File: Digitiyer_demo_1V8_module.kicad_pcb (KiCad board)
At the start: 2 copper layers, 37.8 x 35 mm, 104 parts, among them J1 Conn_01x08, J2 Conn_01x24, J3 Conn_01x04_Pin, J4 USB_C_Receptacle_PowerOnly_6P, Q1 AO3400A, Q2 SI1308EDL, U1 Opamp_Quad, U2 LM27762DSSR, U3 TMUX1108PWR, U4 RF-BM-ND05, U5 TPS63900DSKR, U6 TXB0108PWR, U7 74LVC1G34GW, U8 74LVC1G34GW

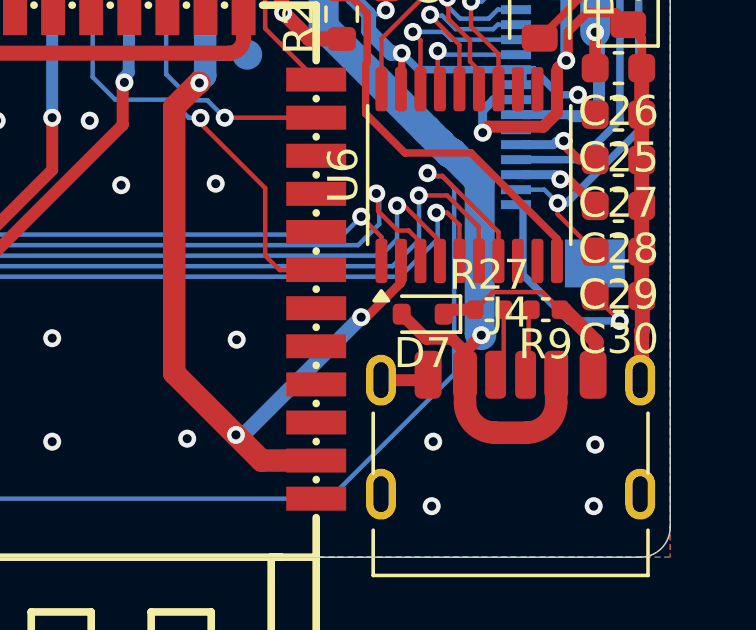
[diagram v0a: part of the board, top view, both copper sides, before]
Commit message: uložit
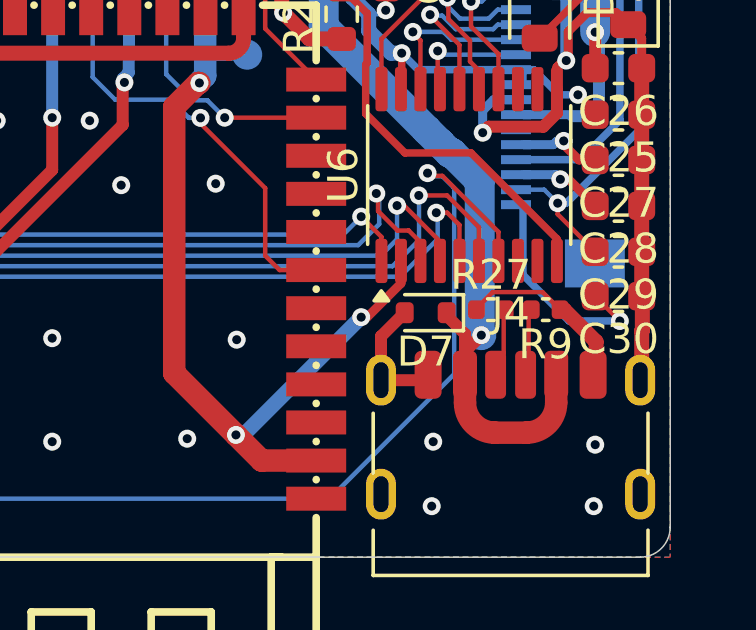
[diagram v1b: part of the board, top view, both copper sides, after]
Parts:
- moved D7 0.11 mm to (181.3, 92.8)
- moved R27 0.05 mm to (183.5, 92.8)
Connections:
- C35 pad 2: Net-(D7-A) -> Net-(D7-C)
- D7 pad 1: GND -> Net-(D7-C)
- D7 pad 2: Net-(D7-A) -> GND
- J4 pad A9: Net-(D7-A) -> Net-(D7-C)
- J4 pad B9: Net-(D7-A) -> Net-(D7-C)
- U5 pad 1: Net-(D7-A) -> Net-(D7-C)
- U5 pad 10: Net-(D7-A) -> Net-(D7-C)
- U5 pad 2: Net-(D7-A) -> Net-(D7-C)
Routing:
- net Net-(D7-A): track 39.4 -> 0.00 mm, vias 2 -> 0
- net Net-(D7-C): track 0.00 -> 38.3 mm, vias 0 -> 2
- net GND: track 107.0 -> 108.6 mm
